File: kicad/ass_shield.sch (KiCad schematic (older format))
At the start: 150 parts, among them J1 6-40V, J2 DEBUG, J3 5V, J4 UART2, J5 U.FL, J7 SP, J8 U.FL, M1 CR1220SMD, Q1 BC817, U1 OPiZero, U2 DS3231M, U3 24LC256, U4 nRF24L01P, U5 PCF8574, U6 CC2530F, X1 USB_F1, X2 USB_F1, Y1 9,84375 MHz, Y2 13,5600 MHz, Y3 4,8970 MHz, Y4 6,7458 MHz, Y5 32 MHz, Y6 16 MHz, Y7 32 MHz

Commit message: Add files via upload
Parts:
- D10, D11, D12, D15, D16, D17, D2, D3, D4, D5, D6, D7: symbol imm_lib:WS2812B -> ass_shield-rescue:WS2812B-imm_lib
- D13, D14: symbol imm_lib:syn470r -> ass_shield-rescue:syn470r-imm_lib
- D8, D9: symbol imm_lib:syn115 -> ass_shield-rescue:syn115-imm_lib
- U1: footprint imm:OPiZero -> imm:OPiZero4
- X1, X2: symbol imm_lib:USB_F1 -> ass_shield-rescue:USB_F1-imm_lib
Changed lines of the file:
@@
 F 0 "U1" H 2175 4147 60  0000 C CNN
 F 1 "OPiZero" H 2175 4041 60  0000 C CNN
-F 2 "imm:OPiZero" H 2200 1500 60  0001 C CNN
+F 2 "imm:OPiZero4" H 2200 1500 60  0001 C CNN
 F 3 "/home/user/kicad/libraries/imm_lib/orange-pi-zero-piout.png" H 2200 1600 60  0001 C CNN
 	1    2200 2350
@@
 $EndComp
 $Comp
-L imm_lib:syn115 D9
+L ass_shield-rescue:syn115-imm_lib D9
 U 1 1 5B6E36AC
 P 2200 7300
@@
 $EndComp
 $Comp
-L imm_lib:syn470r D13
+L ass_shield-rescue:syn470r-imm_lib D13
 U 1 1 5B6E371D
 P 2350 5050
@@
 Connection ~ 850  7350
 $Comp
-L imm_lib:syn115 D8
+L ass_shield-rescue:syn115-imm_lib D8
 U 1 1 5B6E4624
 P 2200 5850
@@
 5V
 $Comp
-L imm_lib:syn470r D14
+L ass_shield-rescue:syn470r-imm_lib D14
 U 1 1 5B70BDEF
 P 2350 6500
@@
 1RF433
 $Comp
-L imm_lib:USB_F1 X1
+L ass_shield-rescue:USB_F1-imm_lib X1
 U 1 1 5B6FAC0C
 P 650 800
@@
 $EndComp
 $Comp
-L imm_lib:USB_F1 X2
+L ass_shield-rescue:USB_F1-imm_lib X2
 U 1 1 5B6FACB0
 P 650 1400
@@
 CE
 $Comp
-L imm_lib:WS2812B D2
+L ass_shield-rescue:WS2812B-imm_lib D2
 U 1 1 5B706A5C
 P 1050 3650
@@
 $EndComp
 $Comp
-L imm_lib:WS2812B D5
+L ass_shield-rescue:WS2812B-imm_lib D5
 U 1 1 5B706C84
 P 1700 3650
@@
 $EndComp
 $Comp
-L imm_lib:WS2812B D10
+L ass_shield-rescue:WS2812B-imm_lib D10
 U 1 1 5B706D18
 P 2350 3650
@@
 $EndComp
 $Comp
-L imm_lib:WS2812B D15
+L ass_shield-rescue:WS2812B-imm_lib D15
 U 1 1 5B706DB2
 P 3000 3650
@@
 $EndComp
 $Comp
-L imm_lib:WS2812B D3
+L ass_shield-rescue:WS2812B-imm_lib D3
 U 1 1 5B706E52
 P 1050 4100
@@
 $EndComp
 $Comp
-L imm_lib:WS2812B D6
+L ass_shield-rescue:WS2812B-imm_lib D6
 U 1 1 5B706F16
 P 1700 4100
@@
 $EndComp
 $Comp
-L imm_lib:WS2812B D11
+L ass_shield-rescue:WS2812B-imm_lib D11
 U 1 1 5B70732F
 P 2350 4100
@@
 $EndComp
 $Comp
-L imm_lib:WS2812B D16
+L ass_shield-rescue:WS2812B-imm_lib D16
 U 1 1 5B7073D5
 P 3000 4100
@@
 	4150 7650 4150 7200
 $Comp
-L imm_lib:WS2812B D4
+L ass_shield-rescue:WS2812B-imm_lib D4
 U 1 1 5BCACDDF
 P 1050 4550
@@
 $EndComp
 $Comp
-L imm_lib:WS2812B D7
+L ass_shield-rescue:WS2812B-imm_lib D7
 U 1 1 5BCACF33
 P 1700 4550
@@
 $EndComp
 $Comp
-L imm_lib:WS2812B D12
+L ass_shield-rescue:WS2812B-imm_lib D12
 U 1 1 5BCAD06D
 P 2350 4550
@@
 $EndComp
 $Comp
-L imm_lib:WS2812B D17
+L ass_shield-rescue:WS2812B-imm_lib D17
 U 1 1 5BDA0DCC
 P 3000 4550

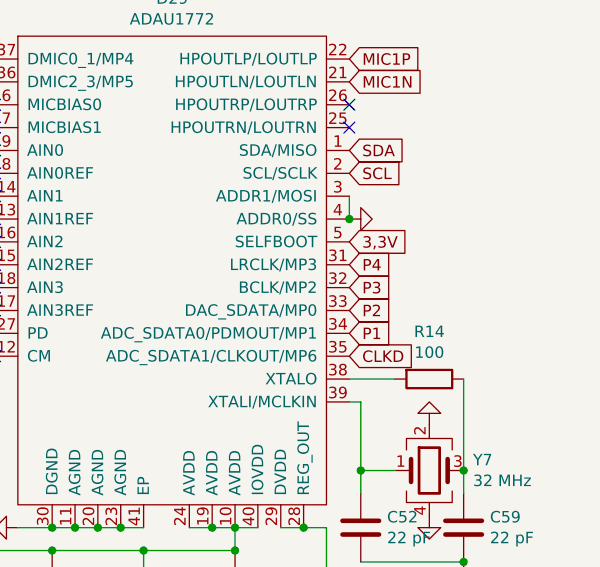
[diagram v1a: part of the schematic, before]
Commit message: Add files via upload
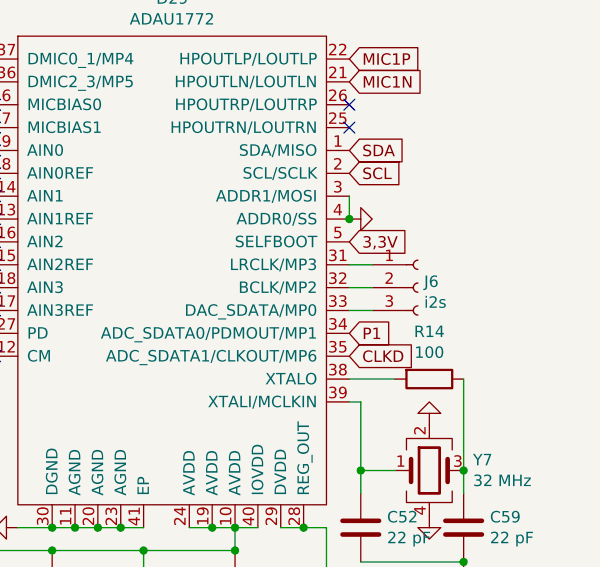
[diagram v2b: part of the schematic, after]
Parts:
- added J6: i2s, Connector_PinSocket_2.54mm:PinSocket_1x03_P2.54mm_Vertical, symbol Connector:Conn_01x03_Female
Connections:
- net P2: no longer D29.33 (DAC_SDATA/MP0)
- net P3: no longer D29.32 (BCLK/MP2)
- net P4: no longer D29.31 (LRCLK/MP3)
- new net: D29.31 (LRCLK/MP3), J6.1 (Pin_1)
- new net: D29.32 (BCLK/MP2), J6.2 (Pin_2)
- new net: D29.33 (DAC_SDATA/MP0), J6.3 (Pin_3)
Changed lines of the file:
@@
 Text GLabel 10300 5000 2    50   Input ~ 0
 P1
-Text GLabel 10300 4900 2    50   Input ~ 0
-P2
-Text GLabel 10300 4800 2    50   Input ~ 0
-P3
-Text GLabel 10300 4700 2    50   Input ~ 0
-P4
 Text GLabel 6800 4950 2    50   Input ~ 0
 P1
@@
 	-1   0    0    1
 $EndComp
+$Comp
+L Connector:Conn_01x03_Female J6
+U 1 1 5B8EB8EC
+P 10600 4800
+F 0 "J6" H 10627 4826 50  0000 L CNN
+F 1 "i2s" H 10627 4735 50  0000 L CNN
+F 2 "Connector_PinSocket_2.54mm:PinSocket_1x03_P2.54mm_Vertical" H 10600 4800 50  0001 C CNN
+F 3 "~
+" H 10600 4800 50  0001 C CNN
+	1    10600 4800
+	1    0    0    -1
+$EndComp
+Wire Wire Line
+	10300 4700 10400 4700
+Wire Wire Line
+	10300 4800 10400 4800
+Wire Wire Line
+	10300 4900 10400 4900
 $EndSCHEMATC
